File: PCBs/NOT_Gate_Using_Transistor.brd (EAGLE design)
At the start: 28 x 26.8 mm, 11 parts, among them T1 BC547, T2 BC547

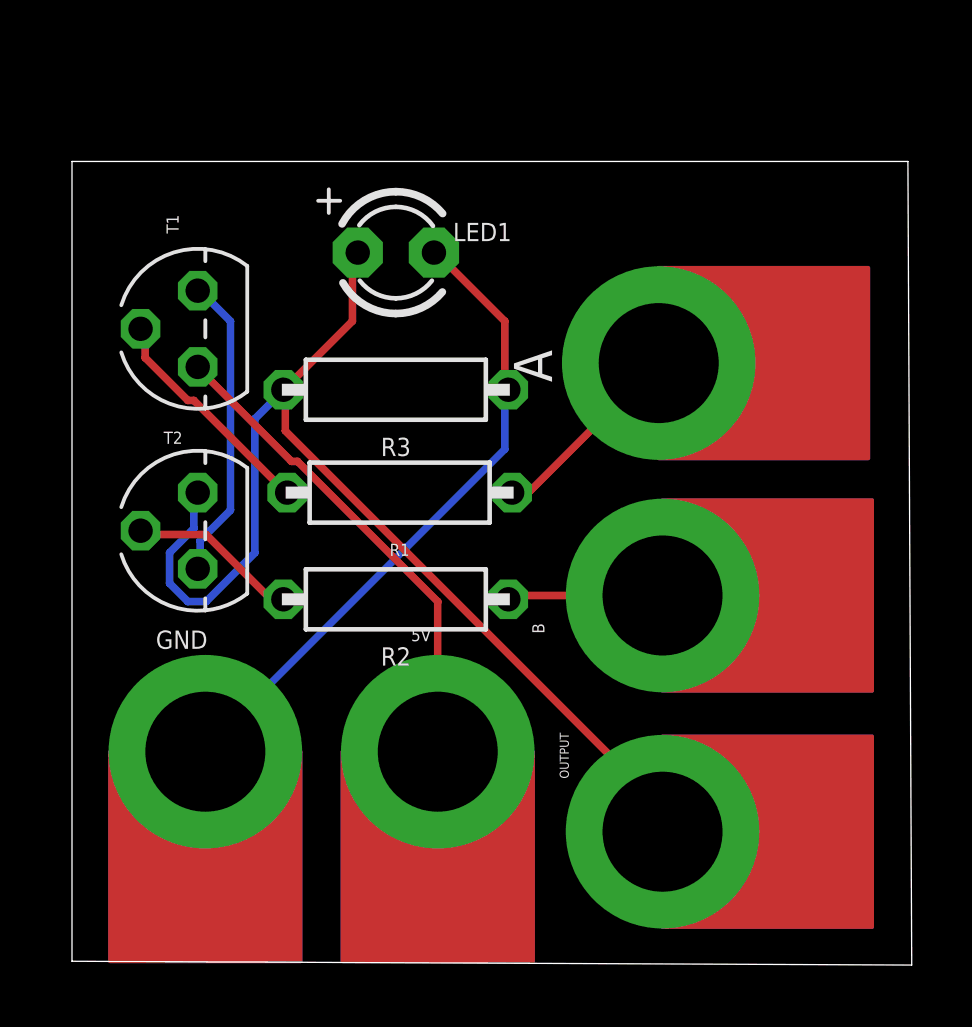
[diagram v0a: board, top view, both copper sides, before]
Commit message: Renamed files .
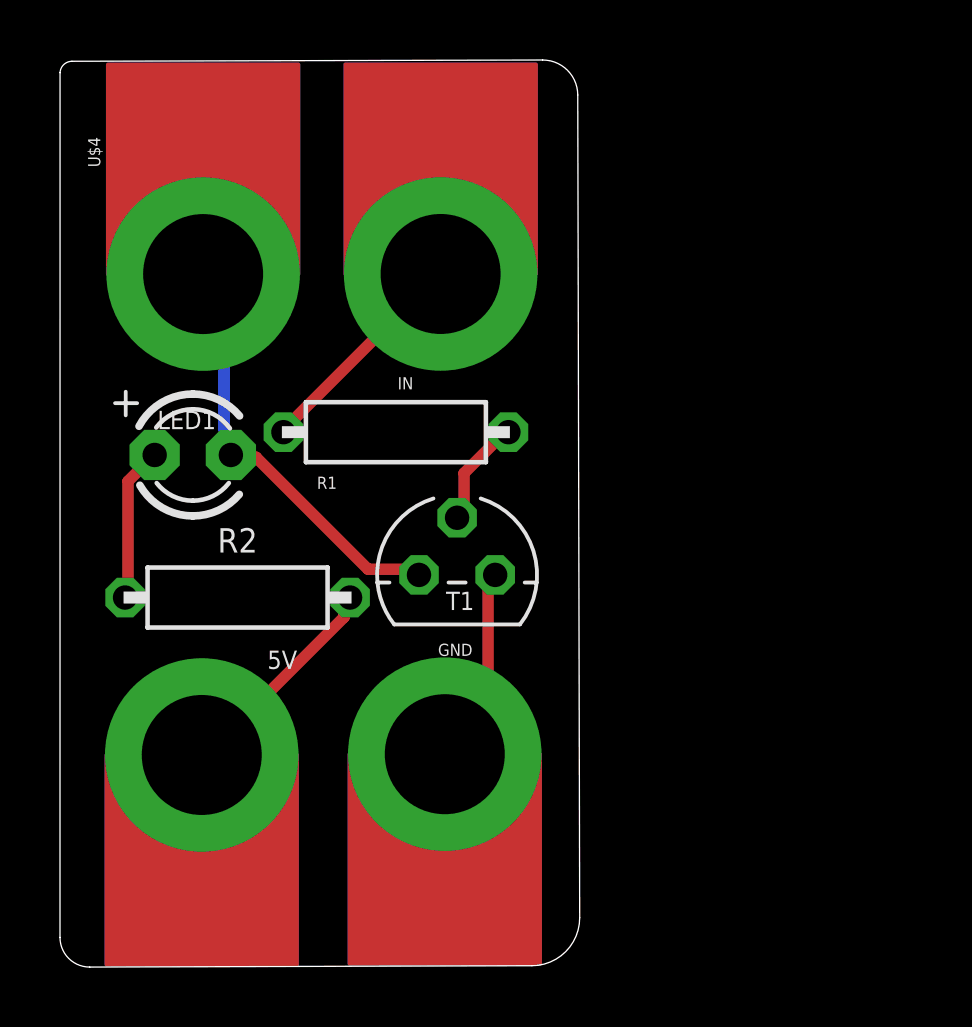
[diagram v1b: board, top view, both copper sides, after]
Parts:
- removed A, B, OUTPUT: MICROBIT_PAD, microbit:MICROBIT_PAD
- removed R3: (no value), we-rcl:R0207/7
- removed T2: BC547, transistor-neu-to92:TO92
- added IN, U$4: MICROBIT_PAD, microbit:MICROBIT_PAD
- R1: value (none) -> 10k
- R2: value (none) -> 470
- T1: device transistor-neu-to92:TO92 -> transistor:TO92
- moved T1 11.9 mm to (12.8, 12.9), turned to 0 degrees
- moved LED1 9.56 mm to (4.03, 16.9)
- moved GND 7.98 mm to (12.4, 6.90)
- moved 5V 7.87 mm to (4.33, 6.88)
- moved R2 5.28 mm to (5.52, 12.1), turned to 0 degrees
- moved R1 2.02 mm to (10.8, 17.6), turned to 0 degrees
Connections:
- removed net N$1 (its old number): R2.2, T2.2
- removed net N$2: T1.1, T2.3
- removed net N$6: A.PAD, R1.1
- removed net N$7: B.PAD, R2.1
- new net N$4: IN.PAD, R1.1
- new net VOUT: LED1.K, T1.3, U$4.PAD
- net 5V: now also R2.2; no longer T1.3
- net GND: now also T1.1; no longer LED1.K, R3.1
- net N$3: now also R2.1; no longer OUTPUT.PAD, R3.2, T2.1
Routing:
- net N$3: track 38.6 -> 5.16 mm
- net GND: track 21.9 -> 6.78 mm
- net VOUT: track 0.00 -> 14.4 mm
- net N$2: track 10.2 -> 0.00 mm
- net 5V: track 16.3 -> 7.40 mm
- net N$4: track 0.00 -> 7.48 mm
- net N$6: track 6.66 -> 0.00 mm
- net N$1 (its old number): track 5.70 -> 0.00 mm
- net N$7: track 5.21 -> 0.00 mm
- net N$1: track 7.62 -> 3.65 mm
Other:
- board size 28 x 26.8 mm -> 17.3 x 30.2 mm
